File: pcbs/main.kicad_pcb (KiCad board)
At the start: 2 copper layers, 261.1 x 103.7 mm, 91 parts

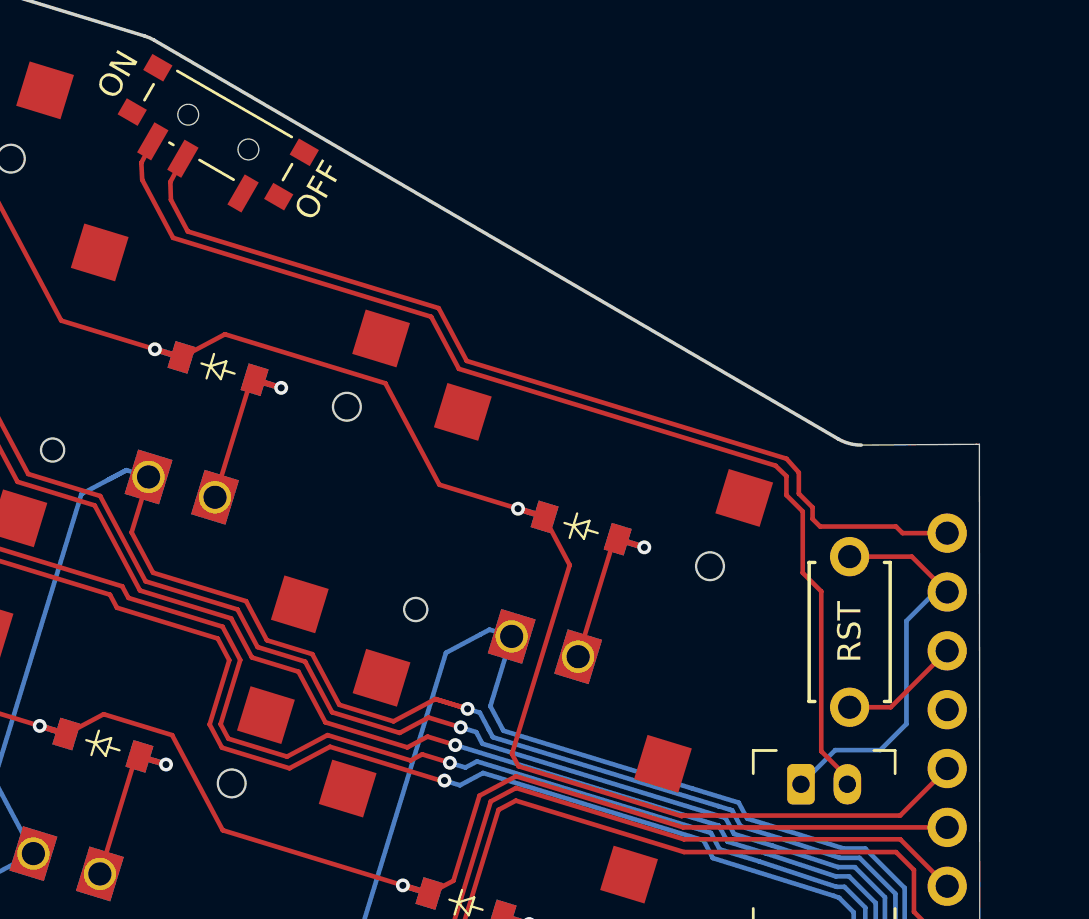
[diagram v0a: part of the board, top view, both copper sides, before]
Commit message: minor changes to the pcb files
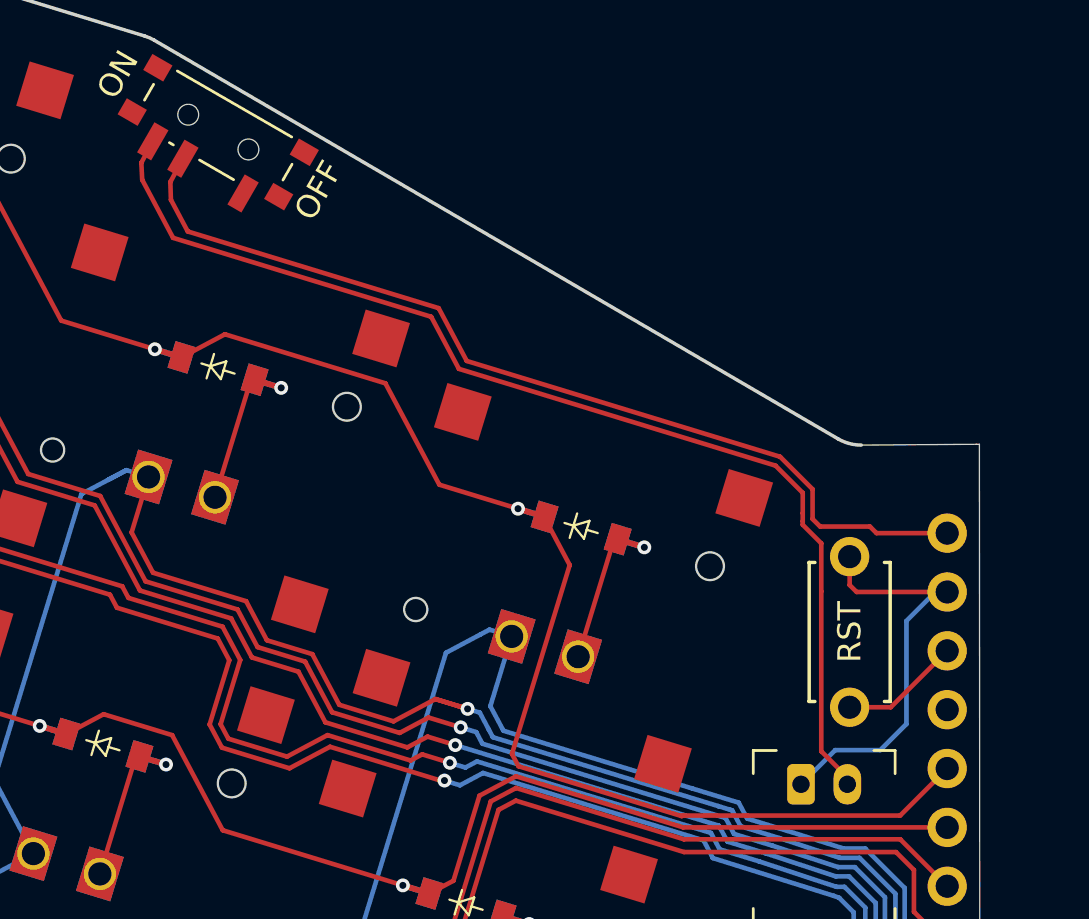
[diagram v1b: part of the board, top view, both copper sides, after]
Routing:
- net GND: track 16.7 -> 17.4 mm
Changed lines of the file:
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@@
+	)
+	(segment
+		(start 168.235005 107.835005)
+		(end 167.95 107.55)
+		(width 0.2)
+		(layer "F.Cu")
+		(net 57)
+	)
+	(segment
+		(start 167.95 107.55)
+		(end 165.800005 107.550005)
+		(width 0.2)
+		(layer "F.Cu")
+		(net 57)
+	)
+	(segment
+		(start 171.284991 107.835005)
+		(end 168.235005 107.835005)
+		(width 0.2)
+		(layer "F.Cu")
+		(net 57)
+	)
+	(segment
+		(start 165.800005 107.550005)
+		(end 165.475006 107.225001)
+		(width 0.2)
+		(layer "F.Cu")
+		(net 57)
+	)
+	(segment
+		(start 165.475006 107.225001)
+		(end 165.475006 105.938748)
+		(width 0.2)
+		(layer "F.Cu")
+		(net 57)
+	)
+	(segment
+		(start 164.075 104.538742)
+		(end 150.548186 100.403171)
+		(width 0.2)
+		(layer "F.Cu")
+		(net 57)
+	)
+	(segment
+		(start 150.548186 100.403171)
+		(end 149.336522 98.124327)
+		(width 0.2)
+		(layer "F.Cu")
+		(net 57)
+	)
+	(segment
+		(start 165.475006 105.938748)
+		(end 164.075 104.538742)
+		(width 0.2)
+		(layer "F.Cu")
+		(net 57)
 	)
 	(segment
@@
 	)
 	(segment
-		(start 164.881187 105.218819)
-		(end 164.349994 104.622816)
-		(width 0.2)
-		(layer "F.Cu")
-		(net 57)
-	)
-	(segment
-		(start 171.285005 107.834994)
-		(end 169.359997 107.835006)
+		(start 137.779249 93.445749)
+		(end 137.755354 92.680348)
+		(width 0.2)
+		(layer "F.Cu")
+		(net 57)
+	)
+	(segment
+		(start 149.336522 98.124327)
+		(end 138.530273 94.820532)
 		(width 0.2)
 		(layer "F.Cu")
@@
 	)
 	(segment
-		(start 137.779249 93.445749)
-		(end 137.755354 92.680348)
-		(width 0.2)
-		(layer "F.Cu")
-		(net 57)
-	)
-	(segment
-		(start 164.881171 106.131185)
-		(end 164.881187 105.218819)
-		(width 0.2)
-		(layer "F.Cu")
-		(net 57)
-	)
-	(segment
-		(start 149.336522 98.124327)
-		(end 138.530273 94.820532)
-		(width 0.2)
-		(layer "F.Cu")
-		(net 57)
-	)
-	(segment
-		(start 169.075 107.549997)
-		(end 165.800005 107.550005)
-		(width 0.2)
-		(layer "F.Cu")
-		(net 57)
-	)
-	(segment
-		(start 164.349994 104.622816)
-		(end 150.548186 100.403171)
-		(width 0.2)
-		(layer "F.Cu")
-		(net 57)
-	)
-	(segment
-		(start 165.800005 107.550005)
-		(end 165.475006 107.225001)
-		(width 0.2)
-		(layer "F.Cu")
-		(net 57)
-	)
-	(segment
-		(start 165.475008 106.725006)
-		(end 164.881171 106.131185)
-		(width 0.2)
-		(layer "F.Cu")
-		(net 57)
-	)
-	(segment
-		(start 150.548186 100.403171)
-		(end 149.336522 98.124327)
-		(width 0.2)
-		(layer "F.Cu")
-		(net 57)
-	)
-	(segment
-		(start 169.359997 107.835006)
-		(end 169.075 107.549997)
-		(width 0.2)
-		(layer "F.Cu")
-		(net 57)
-	)
-	(segment
-		(start 165.475006 107.225001)
-		(end 165.475008 106.725006)
-		(width 0.2)
-		(layer "F.Cu")
-		(net 57)
-	)
-	(segment
 		(start 138.530273 94.820532)
 		(end 138.506359 94.813236)
@@
 	)
 	(segment
-		(start 167.075001 108.85)
-		(end 169.76001 108.850005)
-		(width 0.2)
-		(layer "F.Cu")
-		(net 58)
-	)
-	(segment
-		(start 169.76001 108.850005)
-		(end 171.284992 110.374985)
+		(start 167.075006 108.850003)
+		(end 167.075006 110.075006)
+		(width 0.2)
+		(layer "F.Cu")
+		(net 58)
+	)
+	(segment
+		(start 167.374988 110.374988)
+		(end 171.284993 110.374988)
+		(width 0.2)
+		(layer "F.Cu")
+		(net 58)
+	)
+	(segment
+		(start 167.075006 110.075006)
+		(end 167.374988 110.374988)
 		(width 0.2)
 		(layer "F.Cu")
@@
 	)
 	(segment
+		(start 165.050002 107.475002)
+		(end 165.850003 108.275003)
+		(width 0.2)
+		(layer "F.Cu")
+		(net 65)
+	)
+	(segment
+		(start 136.997404 90.924214)
+		(end 136.502864 91.852867)
+		(width 0.2)
+		(layer "F.Cu")
+		(net 65)
+	)
+	(segment
+		(start 137.87274 95.090079)
+		(end 149.013686 98.496203)
+		(width 0.2)
+		(layer "F.Cu")
+		(net 65)
+	)
+	(segment
+		(start 165.850008 117.25)
+		(end 166.974993 118.374999)
+		(width 0.2)
+		(layer "F.Cu")
+		(net 65)
+	)
+	(segment
+		(start 165.850003 108.275003)
+		(end 165.850003 110.349996)
+		(width 0.2)
+		(layer "F.Cu")
+		(net 65)
+	)
+	(segment
+		(start 149.013686 98.496203)
+		(end 150.208769 100.743818)
+		(width 0.2)
+		(layer "F.Cu")
+		(net 65)
+	)
+	(segment
+		(start 150.208769 100.743818)
+		(end 163.875 104.922003)
+		(width 0.2)
+		(layer "F.Cu")
+		(net 65)
+	)
+	(segment
 		(start 163.875 104.922003)
-		(end 164.346124 105.374995)
-		(width 0.2)
-		(layer "F.Cu")
-		(net 65)
-	)
-	(segment
-		(start 165.850008 117.25)
-		(end 165.850003 110.349996)
-		(width 0.2)
-		(layer "F.Cu")
-		(net 65)
-	)
-	(segment
-		(start 164.346124 105.374995)
-		(end 164.346132 106.19612)
+		(end 165.050004 106.097007)
+		(width 0.2)
+		(layer "F.Cu")
+		(net 65)
+	)
+	(segment
+		(start 165.050002 107.325)
+		(end 165.050002 107.475002)
 		(width 0.2)
 		(layer "F.Cu")
@@
 	)
 	(segment
-		(start 136.502864 91.852867)
-		(end 136.997404 90.924214)
+		(start 165.050004 106.975)
+		(end 165.050002 107.325)
 		(width 0.2)
 		(layer "F.Cu")
@@
 	)
 	(segment
-		(start 165.049992 109.549993)
-		(end 165.850003 110.349996)
-		(width 0.2)
-		(layer "F.Cu")
-		(net 65)
-	)
-	(segment
-		(start 166.974993 118.374999)
+		(start 165.850003 110.349996)
 		(end 165.850008 117.25)
 		(width 0.2)
@@
 	)
 	(segment
-		(start 137.87274 95.090079)
-		(end 149.013686 98.496203)
-		(width 0.2)
-		(layer "F.Cu")
-		(net 65)
-	)
-	(segment
-		(start 165.050004 106.89999)
-		(end 165.049992 109.549993)
-		(width 0.2)
-		(layer "F.Cu")
-		(net 65)
-	)
-	(segment
-		(start 164.346132 106.19612)
-		(end 165.050004 106.89999)
-		(width 0.2)
-		(layer "F.Cu")
-		(net 65)
-	)
-	(segment
-		(start 150.208769 100.743818)
-		(end 163.875 104.922003)
-		(width 0.2)
-		(layer "F.Cu")
-		(net 65)
-	)
-	(segment
-		(start 149.013686 98.496203)
-		(end 150.208769 100.743818)
-		(width 0.2)
-		(layer "F.Cu")
+		(start 165.050004 106.097007)
+		(end 165.050004 106.975)
+		(width 0.2)
+		(layer "F.Cu")
